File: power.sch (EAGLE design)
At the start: 37 parts, among them CN1 21700, CN2 21700, CN3 21700, CN4 21700, CN5 15PIN 0.5MM, Q1 IRLML6244, Q2 IRLML6244, U1 MAX17320G20+

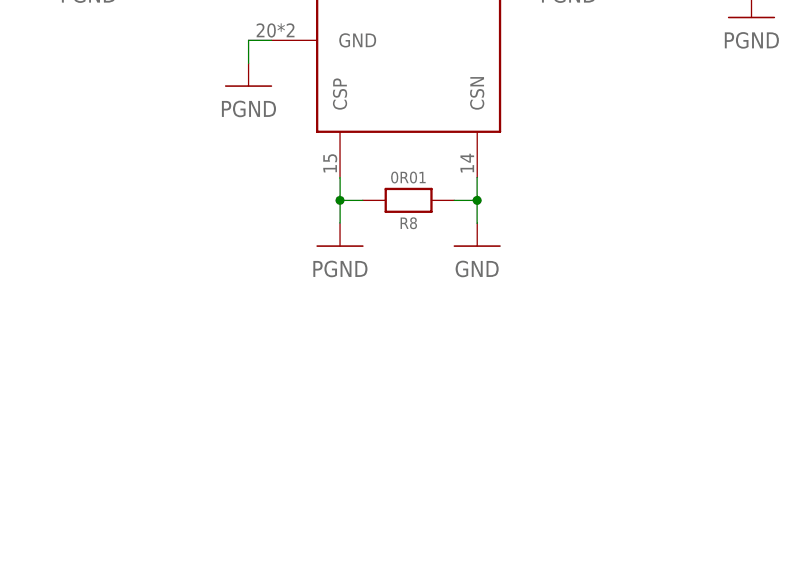
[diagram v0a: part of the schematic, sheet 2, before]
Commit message: debug board done
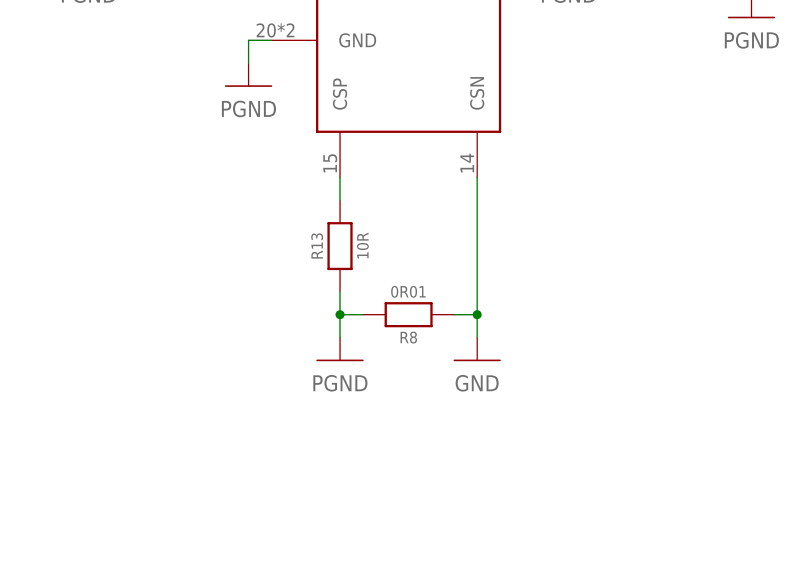
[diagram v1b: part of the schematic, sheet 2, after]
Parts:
- added R13: 10R, r_0603:ERJ3EKF10R0V
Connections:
- new net N$6: R13.2, U1.CSP
- net PGND: now also R13.1; no longer U1.CSP
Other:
- moved on the sheet: R8
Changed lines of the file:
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@@
 <part name="MECH6" library="MISC" deviceset="MOUNTHOLE" device="" value="6mm x 3mm"/>
 <part name="U$2" library="NETS" deviceset="PGND" device=""/>
+<part name="R13" library="r_0603" deviceset="ERJ3EKF10R0V" device="" value="10R"/>
 </parts>
 <sheets>
@@
 <attribute name="VALUE" x="-33.02" y="7.62" size="1.27" layer="96" rot="R90" align="center"/>
 </instance>
-<instance part="R8" gate="G$1" x="0" y="-73.66" smashed="yes" rot="R180">
-<attribute name="NAME" x="0" y="-76.2" size="1.27" layer="95" rot="R180" align="center"/>
-<attribute name="VALUE" x="0" y="-71.12" size="1.27" layer="96" rot="R180" align="center"/>
+<instance part="R8" gate="G$1" x="0" y="-86.36" smashed="yes" rot="R180">
+<attribute name="NAME" x="0" y="-88.9" size="1.27" layer="95" rot="R180" align="center"/>
+<attribute name="VALUE" x="0" y="-83.82" size="1.27" layer="96" rot="R180" align="center"/>
 </instance>
 <instance part="C5" gate="G$1" x="-30.48" y="30.48" smashed="yes" rot="R90">
@@
 <attribute name="VALUE" x="22.86" y="-2.54" size="1.27" layer="96" align="center"/>
 </instance>
-<instance part="U$20" gate="G$1" x="-7.62" y="-78.74" smashed="yes">
-<attribute name="VALUE" x="-7.62" y="-81.28" size="1.778" layer="96" align="center"/>
-</instance>
-<instance part="GND2" gate="G$1" x="7.62" y="-78.74" smashed="yes">
-<attribute name="VALUE" x="7.62" y="-81.28" size="1.778" layer="96" align="center"/>
+<instance part="U$20" gate="G$1" x="-7.62" y="-91.44" smashed="yes">
+<attribute name="VALUE" x="-7.62" y="-93.98" size="1.778" layer="96" align="center"/>
+</instance>
+<instance part="GND2" gate="G$1" x="7.62" y="-91.44" smashed="yes">
+<attribute name="VALUE" x="7.62" y="-93.98" size="1.778" layer="96" align="center"/>
 </instance>
 <instance part="U$21" gate="G$1" x="-30.48" y="20.32" smashed="yes">
@@
 <instance part="U$2" gate="G$1" x="43.18" y="17.78" smashed="yes">
 <attribute name="VALUE" x="43.18" y="15.24" size="1.778" layer="96" align="center"/>
+</instance>
+<instance part="R13" gate="G$1" x="-7.62" y="-78.74" smashed="yes" rot="R90">
+<attribute name="NAME" x="-10.16" y="-78.74" size="1.27" layer="95" rot="R90" align="center"/>
+<attribute name="VALUE" x="-5.08" y="-78.74" size="1.27" layer="96" rot="R90" align="center"/>
 </instance>
 </instances>
@@
 <segment>
 <pinref part="R8" gate="G$1" pin="1"/>
-<wire x1="5.08" y1="-73.66" x2="7.62" y2="-73.66" width="0.1524" layer="91"/>
+<wire x1="5.08" y1="-86.36" x2="7.62" y2="-86.36" width="0.1524" layer="91"/>
 <pinref part="U1" gate="G$1" pin="CSN"/>
-<wire x1="7.62" y1="-71.12" x2="7.62" y2="-73.66" width="0.1524" layer="91"/>
-<junction x="7.62" y="-73.66"/>
+<wire x1="7.62" y1="-71.12" x2="7.62" y2="-86.36" width="0.1524" layer="91"/>
+<junction x="7.62" y="-86.36"/>
 <pinref part="GND2" gate="G$1" pin="GND"/>
-<wire x1="7.62" y1="-76.2" x2="7.62" y2="-73.66" width="0.1524" layer="91"/>
+<wire x1="7.62" y1="-88.9" x2="7.62" y2="-86.36" width="0.1524" layer="91"/>
 </segment>
 <segment>
@@
 <segment>
 <pinref part="R8" gate="G$1" pin="2"/>
-<wire x1="-5.08" y1="-73.66" x2="-7.62" y2="-73.66" width="0.1524" layer="91"/>
-<pinref part="U1" gate="G$1" pin="CSP"/>
-<wire x1="-7.62" y1="-71.12" x2="-7.62" y2="-73.66" width="0.1524" layer="91"/>
-<junction x="-7.62" y="-73.66"/>
+<wire x1="-5.08" y1="-86.36" x2="-7.62" y2="-86.36" width="0.1524" layer="91"/>
+<junction x="-7.62" y="-86.36"/>
 <pinref part="U$20" gate="G$1" pin="PGND"/>
-<wire x1="-7.62" y1="-76.2" x2="-7.62" y2="-73.66" width="0.1524" layer="91"/>
+<wire x1="-7.62" y1="-88.9" x2="-7.62" y2="-86.36" width="0.1524" layer="91"/>
+<wire x1="-7.62" y1="-83.82" x2="-7.62" y2="-86.36" width="0.1524" layer="91"/>
+<pinref part="R13" gate="G$1" pin="1"/>
 </segment>
 <segment>
@@
 </segment>
 </net>
+<net name="N$6" class="0">
+<segment>
+<pinref part="U1" gate="G$1" pin="CSP"/>
+<wire x1="-7.62" y1="-71.12" x2="-7.62" y2="-73.66" width="0.1524" layer="91"/>
+<pinref part="R13" gate="G$1" pin="2"/>
+</segment>
+</net>
